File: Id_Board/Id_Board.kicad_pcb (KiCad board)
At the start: 2 copper layers, 130 x 50 mm, 2 parts

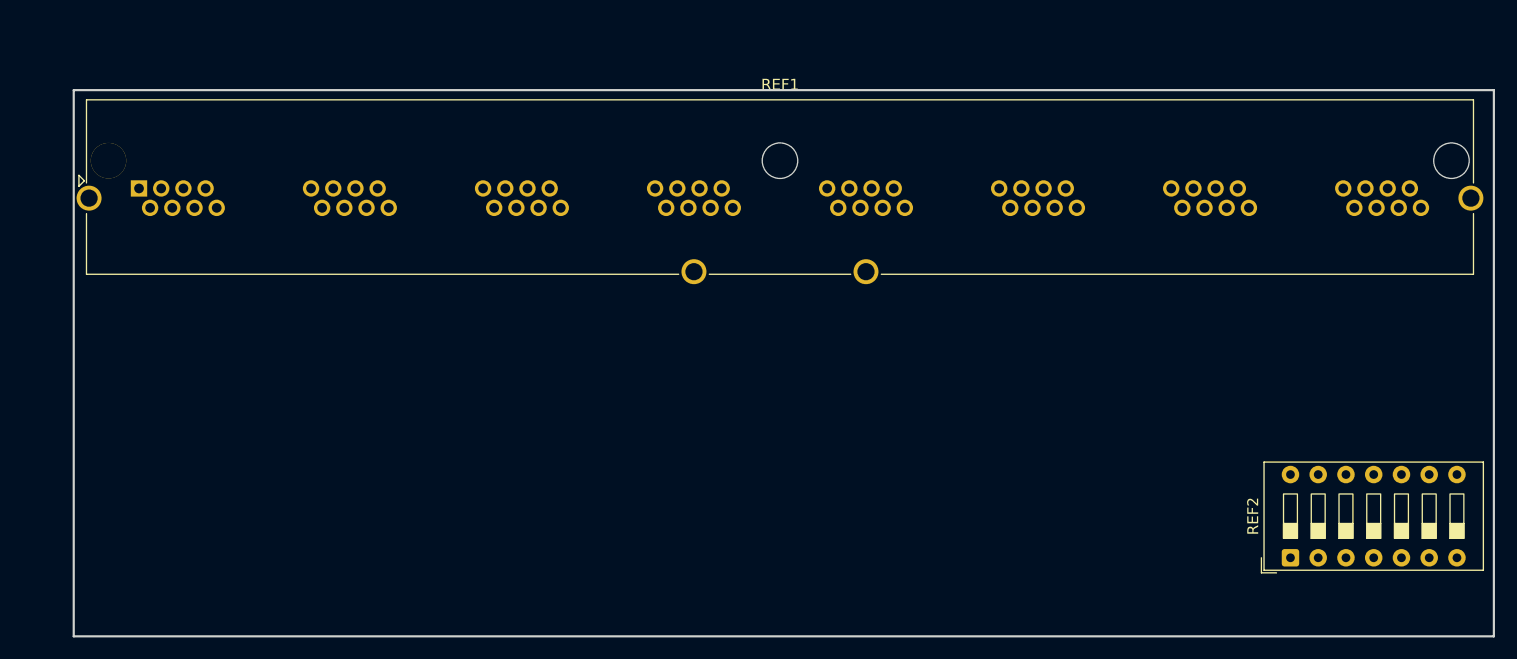
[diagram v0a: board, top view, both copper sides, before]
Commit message: finished IdBoard
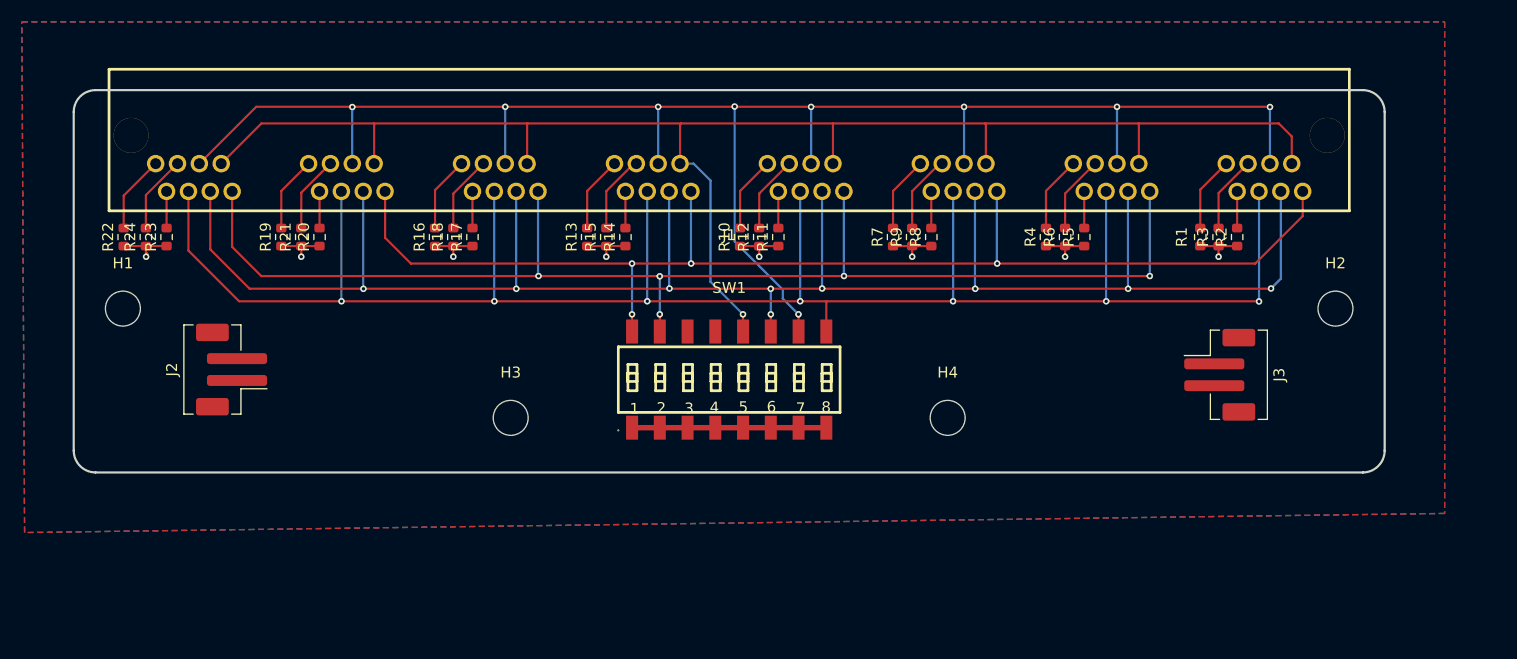
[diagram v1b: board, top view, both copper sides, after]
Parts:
- removed REF1: RJ45_Amphenol_RJHSE5380-08, Connector_RJ:RJ45_Amphenol_RJHSE5380-08
- removed REF2: SW_DIP_SPSTx07_Slide_9.78x19.96mm_W7.62mm_P2.54mm, Button_Switch_THT:SW_DIP_SPSTx07_Slide_9.78x19.96mm_W7.62mm_P2.54mm
- added H1: MountingHole, MountingHole:MountingHole_3.2mm_M3, F.Cu at (64.5, 60.0)
- added H2: MountingHole, MountingHole:MountingHole_3.2mm_M3, F.Cu at (175.5, 60.0)
- added H3: MountingHole, MountingHole:MountingHole_3.2mm_M3, F.Cu at (100.0, 70.0)
- added H4: MountingHole, MountingHole:MountingHole_3.2mm_M3, F.Cu at (140.0, 70.0)
- added J1: ~, LCSC:RJ45-TH_HC-WK88-H13-1X8-55QS_1, F.Cu at (120.0, 48.0)
- added J2: Conn_01x02_Pin, Connector_JST:JST_PH_B2B-PH-SM4-TB_1x02-1MP_P2.00mm_Vertical, F.Cu at (74.4, 65.6)
- added J3: Conn_01x02_Pin, Connector_JST:JST_PH_B2B-PH-SM4-TB_1x02-1MP_P2.00mm_Vertical, F.Cu at (164.9, 66.1)
- added R1: 0, Resistor_SMD:R_0603_1608Metric, F.Cu at (163.1, 53.5)
- added R10: 0, Resistor_SMD:R_0603_1608Metric, F.Cu at (121.0, 53.5)
- added R11: 0, Resistor_SMD:R_0603_1608Metric, F.Cu at (124.5, 53.5)
- added R12: 0, Resistor_SMD:R_0603_1608Metric, F.Cu at (122.8, 53.5)
- added R13: 0, Resistor_SMD:R_0603_1608Metric, F.Cu at (107.0, 53.5)
- added R14: 0, Resistor_SMD:R_0603_1608Metric, F.Cu at (110.5, 53.5)
- added R15: 0, Resistor_SMD:R_0603_1608Metric, F.Cu at (108.8, 53.5)
- added R16: 0, Resistor_SMD:R_0603_1608Metric, F.Cu at (93.1, 53.5)
- added R17: 0, Resistor_SMD:R_0603_1608Metric, F.Cu at (96.5, 53.5)
- added R18: 0, Resistor_SMD:R_0603_1608Metric, F.Cu at (94.8, 53.5)
- added R19: 0, Resistor_SMD:R_0603_1608Metric, F.Cu at (79.0, 53.5)
- added R2: 0, Resistor_SMD:R_0603_1608Metric, F.Cu at (166.5, 53.5)
- added R20: 0, Resistor_SMD:R_0603_1608Metric, F.Cu at (82.5, 53.5)
- added R21: 0, Resistor_SMD:R_0603_1608Metric, F.Cu at (80.8, 53.5)
- added R22: 0, Resistor_SMD:R_0603_1608Metric, F.Cu at (64.6, 53.5)
- added R23: 0, Resistor_SMD:R_0603_1608Metric, F.Cu at (68.5, 53.5)
- added R24: 0, Resistor_SMD:R_0603_1608Metric, F.Cu at (66.6, 53.5)
- added R3: 0, Resistor_SMD:R_0603_1608Metric, F.Cu at (164.8, 53.5)
- added R4: 0, Resistor_SMD:R_0603_1608Metric, F.Cu at (149.0, 53.5)
- added R5: 0, Resistor_SMD:R_0603_1608Metric, F.Cu at (152.5, 53.5)
- added R6: 0, Resistor_SMD:R_0603_1608Metric, F.Cu at (150.8, 53.5)
- added R7: 0, Resistor_SMD:R_0603_1608Metric, F.Cu at (135.0, 53.5)
- added R8: 0, Resistor_SMD:R_0603_1608Metric, F.Cu at (138.5, 53.5)
- added R9: 0, Resistor_SMD:R_0603_1608Metric, F.Cu at (136.8, 53.5)
- added SW1: SW_DIP_x08, LCSC:SW-SMD_16P-L20.3-W6.0-P2.54-LS9.3-BL, F.Cu at (120.0, 66.5)
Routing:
- net BoardA: track 0.00 -> 178.6 mm, vias 0 -> 7
- net BoardC: track 0.00 -> 170.7 mm, vias 0 -> 9
- net BoardB: track 0.00 -> 159.8 mm, vias 0 -> 9
- net BoardD: track 0.00 -> 143.2 mm, vias 0 -> 1
- net ParityB: track 0.00 -> 118.5 mm, vias 0 -> 5
- net ParityA: track 0.00 -> 112.7 mm, vias 0 -> 4
- net GND: track 0.00 -> 52.6 mm, vias 0 -> 8
- net Net-(J1-PadE3): track 0.00 -> 7.27 mm
- net Net-(J1-PadC3): track 0.00 -> 7.17 mm
- net Net-(J1-PadH1): track 0.00 -> 7.11 mm
- net Net-(J1-PadH3): track 0.00 -> 7.10 mm
- net Net-(J1-PadF3): track 0.00 -> 7.04 mm
- net Net-(J1-PadD3): track 0.00 -> 7.04 mm
- net Net-(J1-PadB3): track 0.00 -> 7.04 mm
- net Net-(J1-PadA3): track 0.00 -> 7.02 mm
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- added copper zone on B.Cu, net GND
- added copper zone on F.Cu, net GND
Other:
- board size 130 x 50 mm -> 120 x 35 mm

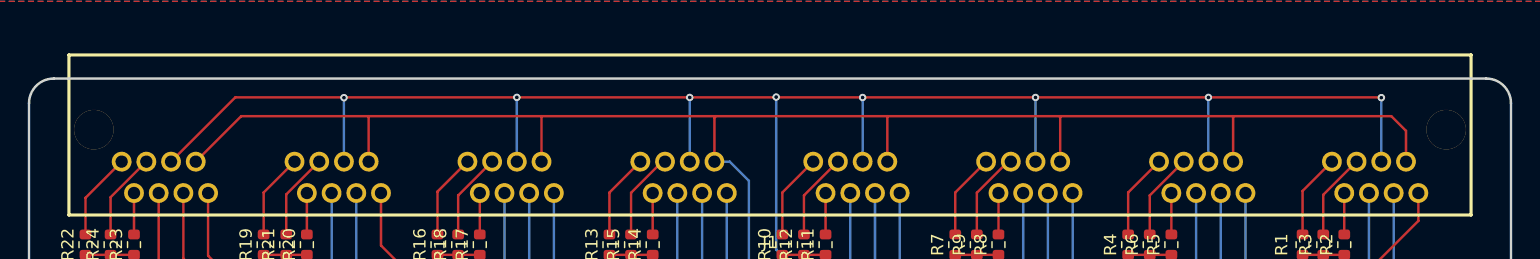
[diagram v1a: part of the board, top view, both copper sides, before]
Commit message: Production File generate
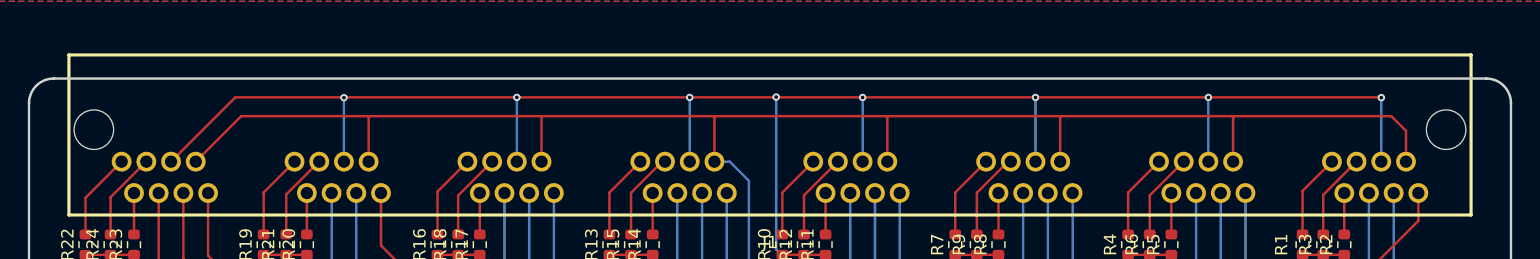
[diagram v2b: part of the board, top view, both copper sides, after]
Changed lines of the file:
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@@
 				(font
 					(size 1.27 1.27)
+					(thickness 0.15)
 				)
 			)
@@
 				(font
 					(size 1.27 1.27)
+					(thickness 0.15)
 				)
 			)
@@
 				(font
 					(size 1.27 1.27)
+					(thickness 0.15)
 				)
 			)
@@
 		(sheetname "/")
 		(sheetfile "Id_Board.kicad_sch")
-		(units
-			(unit
-				(name "A")
-				(pins "A8" "A7" "A6" "A5" "A4" "A3" "A2" "A1")
-			)
-			(unit
-				(name "B")
-				(pins "B8" "B7" "B6" "B5" "B4" "B3" "B2" "B1")
-			)
-			(unit
-				(name "C")
-				(pins "C8" "C7" "C6" "C5" "C4" "C3" "C2" "C1")
-			)
-			(unit
-				(name "D")
-				(pins "D8" "D7" "D6" "D5" "D4" "D3" "D2" "D1")
-			)
-			(unit
-				(name "E")
-				(pins "E8" "E7" "E6" "E5" "E4" "E3" "E2" "E1")
-			)
-			(unit
-				(name "F")
-				(pins "F8" "F7" "F6" "F5" "F4" "F3" "F2" "F1")
-			)
-			(unit
-				(name "G")
-				(pins "G8" "G7" "G6" "G5" "G4" "G3" "G2" "G1")
-			)
-			(unit
-				(name "H")
-				(pins "H8" "H7" "H6" "H5" "H4" "H3" "H2" "H1")
-			)
-		)
 		(attr through_hole)
 		(duplicate_pad_numbers_are_jumpers no)
@@
 			)
 		)
-		(pad "" thru_hole circle
+		(pad "" np_thru_hole circle
 			(at -54.75 3.86 180)
 			(size 3.2 3.2)
 			(drill 3.2)
 			(layers "*.Cu" "*.Mask")
-			(remove_unused_layers no)
 		)
-		(pad "" thru_hole circle
+		(pad "" np_thru_hole circle
 			(at 54.75 3.86 180)
 			(size 3.2 3.2)
 			(drill 3.2)
 			(layers "*.Cu" "*.Mask")
-			(remove_unused_layers no)
 		)
 		(pad "A1" thru_hole circle
@@
 				(font
 					(size 1.27 1.27)
+					(thickness 0.15)
 				)
 			)
@@
 				(font
 					(size 1.27 1.27)
+					(thickness 0.15)
 				)
 			)
@@
 				(font
 					(size 1.27 1.27)
+					(thickness 0.15)
 				)
 			)
@@
 				(font
 					(size 1.27 1.27)
+					(thickness 0.15)
 				)
 			)
@@
 				(font
 					(size 1.27 1.27)
+					(thickness 0.15)
 				)
 			)
@@
 				(font
 					(size 1.27 1.27)
+					(thickness 0.15)
 				)
 			)
@@
 				(font
 					(size 1.27 1.27)
+					(thickness 0.15)
 				)
 			)
@@
 				(font
 					(size 1.27 1.27)
+					(thickness 0.15)
 				)
 			)
@@
 				(font
 					(size 1.27 1.27)
+					(thickness 0.15)
 				)
 			)
@@
 				(font
 					(size 1.27 1.27)
+					(thickness 0.15)
 				)
 			)
@@
 				(font
 					(size 1.27 1.27)
+					(thickness 0.15)
 				)
 			)
@@
 				(font
 					(size 1.27 1.27)
+					(thickness 0.15)
 				)
 			)
@@
 				(font
 					(size 1.27 1.27)
+					(thickness 0.15)
 				)
 			)
@@
 				(font
 					(size 1.27 1.27)
+					(thickness 0.15)
 				)
 			)
@@
 				(font
 					(size 1.27 1.27)
+					(thickness 0.15)
 				)
 			)
@@
 				(font
 					(size 1.27 1.27)
+					(thickness 0.15)
 				)
 			)
@@
 				(font
 					(size 1.27 1.27)
+					(thickness 0.15)
 				)
 			)
@@
 				(font
 					(size 1.27 1.27)
+					(thickness 0.15)
 				)
 			)
@@
 				(font
 					(size 1.27 1.27)
+					(thickness 0.15)
 				)
 			)
@@
 				(font
 					(size 1.27 1.27)
+					(thickness 0.15)
 				)
 			)
@@
 				(font
 					(size 1.27 1.27)
+					(thickness 0.15)
 				)
 			)
